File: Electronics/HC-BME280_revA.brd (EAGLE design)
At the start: 100 x 80 mm, 40 parts, among them SW1 SWITCH_SLIDE, T2 AO3401, U1 ATMEGA328-20P, U2 NRF24L01, U3 BME280, U4 OLED128X64, U5 BCO35

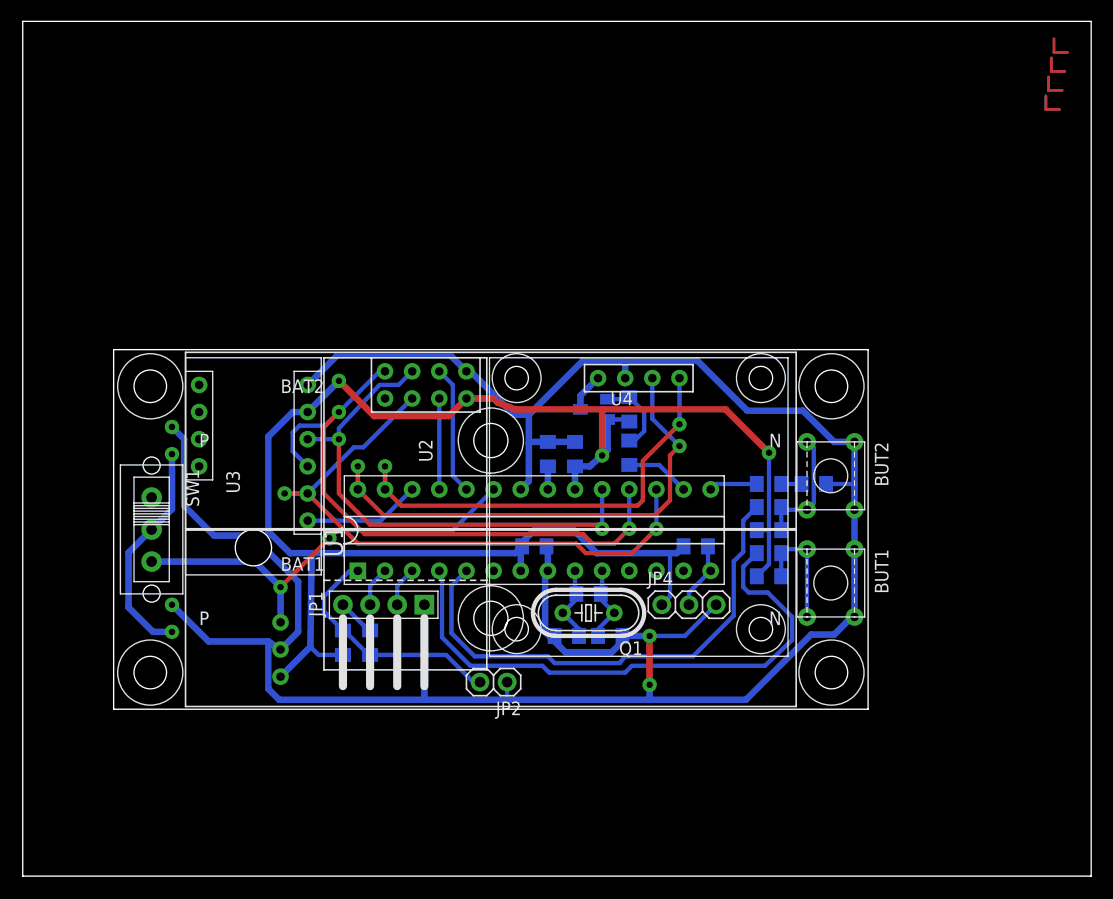
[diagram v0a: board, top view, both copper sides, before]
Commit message: modified: PCB
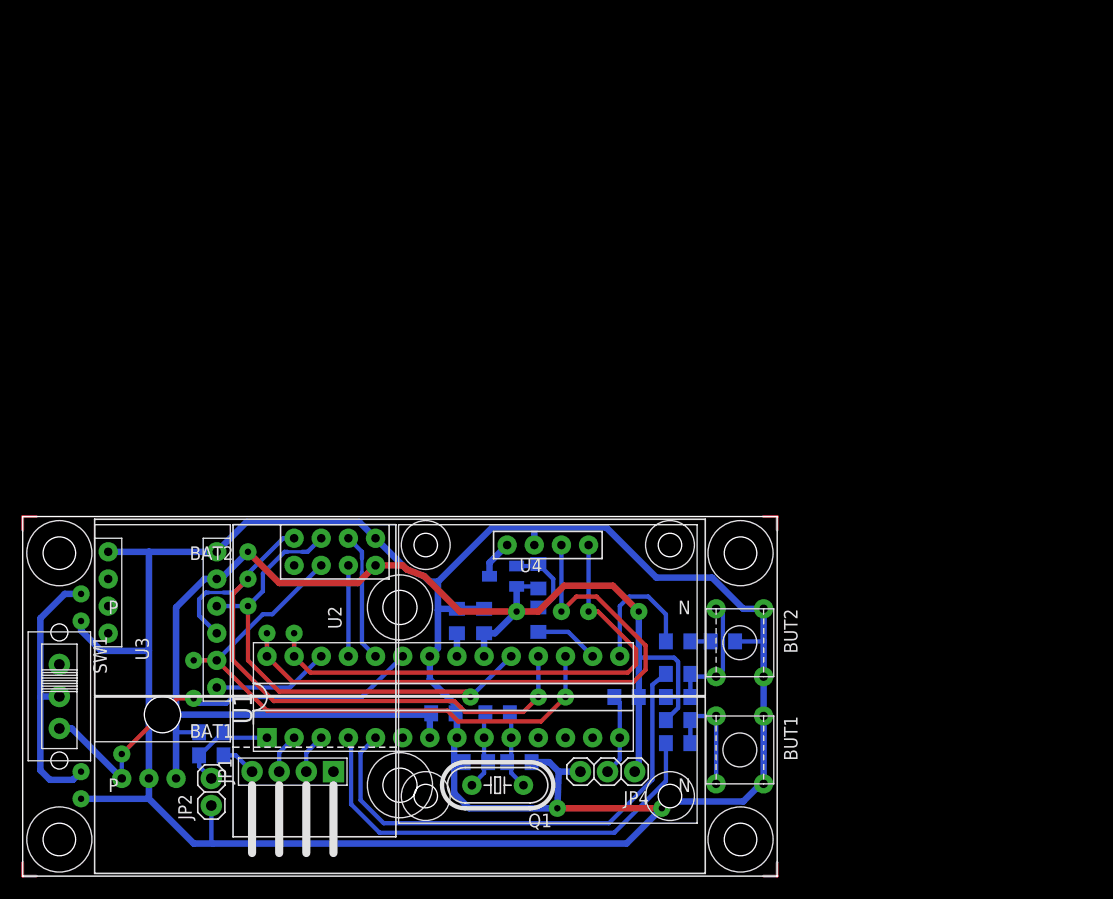
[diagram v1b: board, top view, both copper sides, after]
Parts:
- moved U$2 122.2 mm to (0.64, 0.64)
- moved U$3 104.5 mm to (0.64, 33.0), turned to 270 degrees
- moved U$4 76.5 mm to (70.0, 0.64), turned to 90 degrees
- moved U$1 52.3 mm to (70.0, 33.0), turned to 180 degrees
- moved JP2 28.3 mm to (17.7, 7.87), turned to 90 degrees
- moved R6 19.7 mm to (61.3, 12.4)
- moved Q1 18.2 mm to (44.5, 8.51)
- moved C4 18.2 mm to (17.7, 11.3), turned to 180 degrees
- moved SW1 17.8 mm to (3.43, 16.9)
- moved BAT2 17.8 mm to (35.3, 25.1)
- moved BUT2 17.8 mm to (67.4, 22.5)
- moved R2 17.8 mm to (48.3, 24.0)
- moved R3 17.8 mm to (48.3, 28.1)
- moved T2 17.8 mm to (45.0, 28.1)
- moved U$7 17.8 mm to (3.43, 30.2)
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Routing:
- net +3V3: track 156.0 -> 131.8 mm
- net GND: track 239.6 -> 255.2 mm
- net N$2: track 22.9 -> 10.1 mm
- net SCL: track 48.0 -> 60.1 mm
- net BUT1: track 53.3 -> 42.8 mm
- net SDA: track 42.1 -> 50.8 mm
- net LED: track 4.53 -> 12.6 mm
- net N$8: track 21.0 -> 25.3 mm
- net SCK: track 47.9 -> 46.1 mm
- net DS18B20_1: track 6.41 -> 7.67 mm
- net MISO: track 57.7 -> 58.6 mm
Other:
- board size 100 x 80 mm -> 70.6 x 33.7 mm

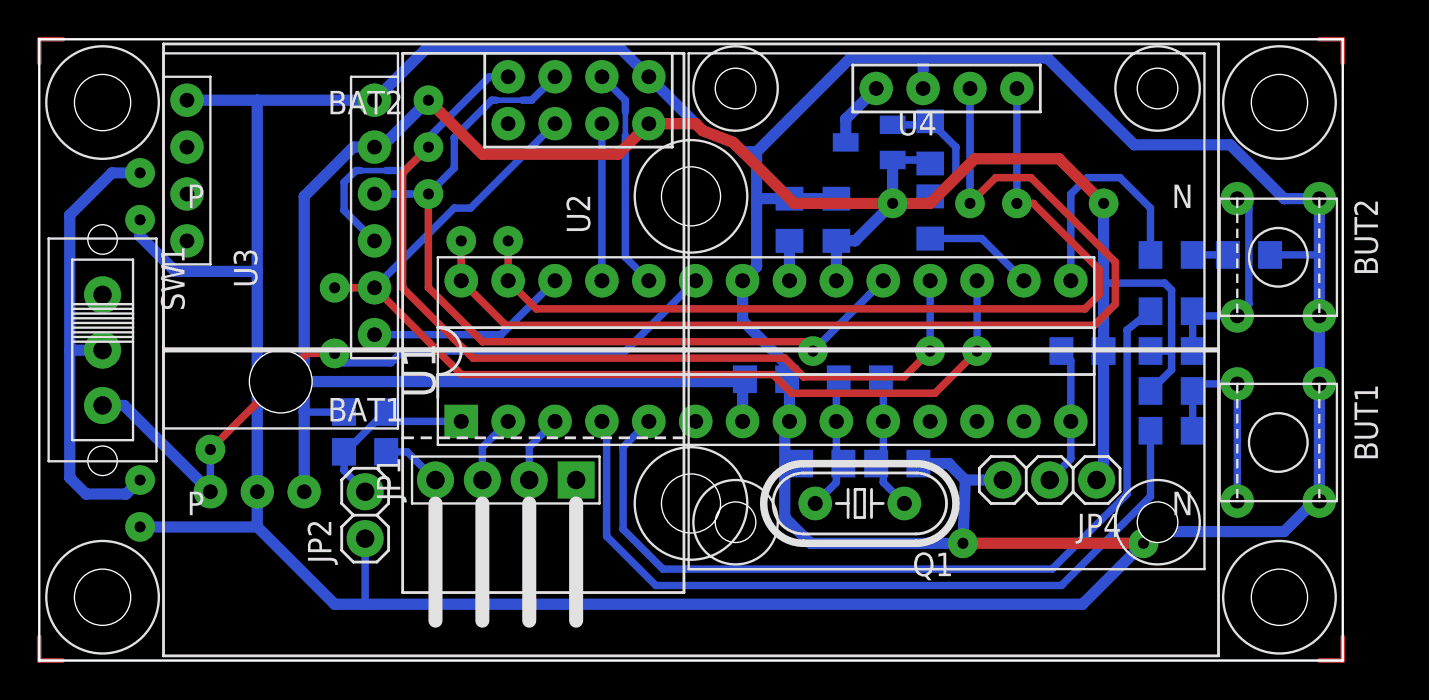
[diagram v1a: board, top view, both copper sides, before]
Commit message: modified: PCB - revA
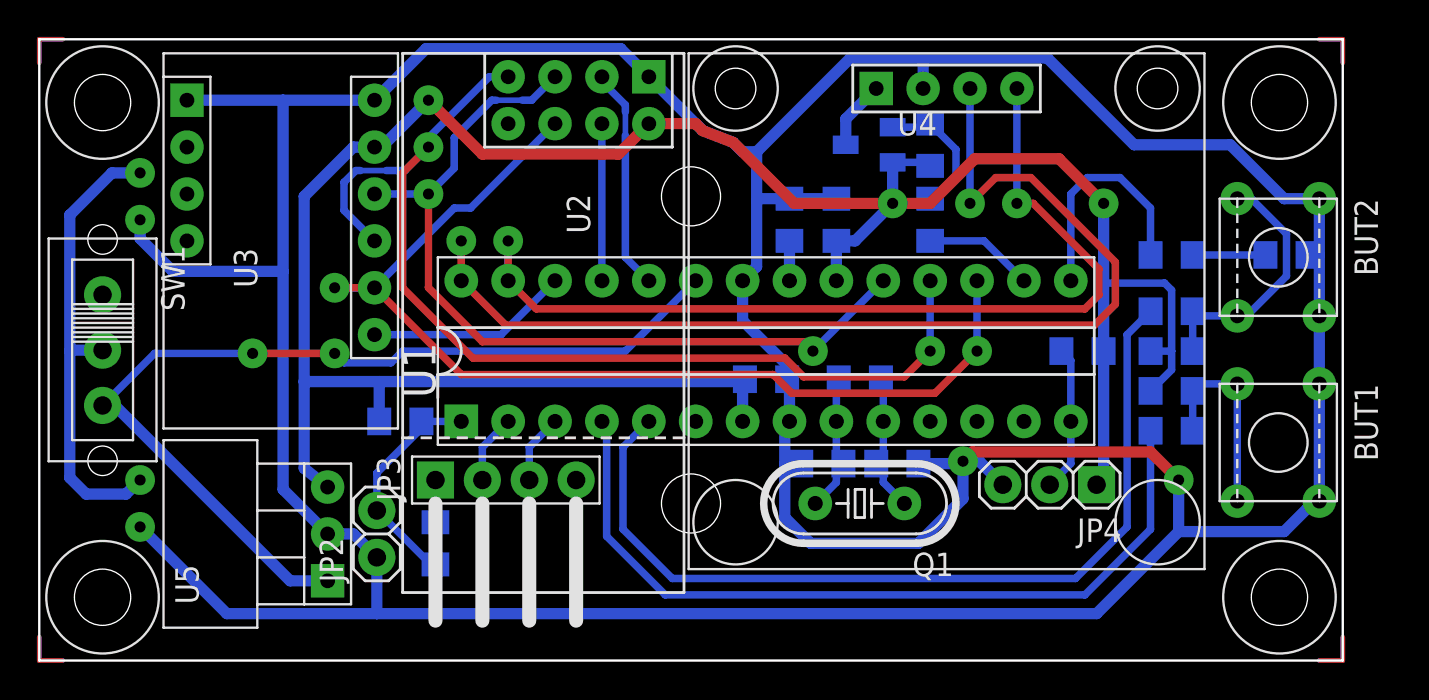
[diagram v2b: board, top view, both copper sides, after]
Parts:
- moved C4 6.25 mm to (21.5, 6.35), turned to 90 degrees
- moved U5 4.44 mm to (15.6, 6.86), flipped to the top, turned to 90 degrees
- moved LED1 2.03 mm to (67.6, 22.0)
- moved R1 1.97 mm to (19.6, 13.0)
- moved JP2 1.20 mm to (18.3, 6.86)
- moved JP4 0.25 mm to (54.7, 9.53)
- moved R2 0.13 mm to (48.3, 23.9)
- moved R3 0.13 mm to (48.3, 27.9)
- moved T2 0.13 mm to (45.0, 27.9)
- flipped BAT1 to the bottom, turned to 180 degrees
- flipped BAT2 to the bottom, turned to 180 degrees
- renumbered JP1 to JP3
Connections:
- net GND: now also JP3.4; no longer JP3.1
- net N$6: now also JP3.1; no longer JP3.4
- net RX: now also JP3.2; no longer JP3.3
- net TX: now also JP3.3; no longer JP3.2
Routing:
- net V_BAT: track 40.6 -> 51.5 mm
- net GND: track 255.2 -> 264.9 mm
- net N$2: track 10.1 -> 12.9 mm
- net N$10: track 11.6 -> 14.0 mm
- net N$11: track 1.90 -> 3.94 mm
- net BUT1: track 42.8 -> 44.3 mm
- net BUT2: track 46.8 -> 48.2 mm
- net N$6: track 3.30 -> 2.29 mm

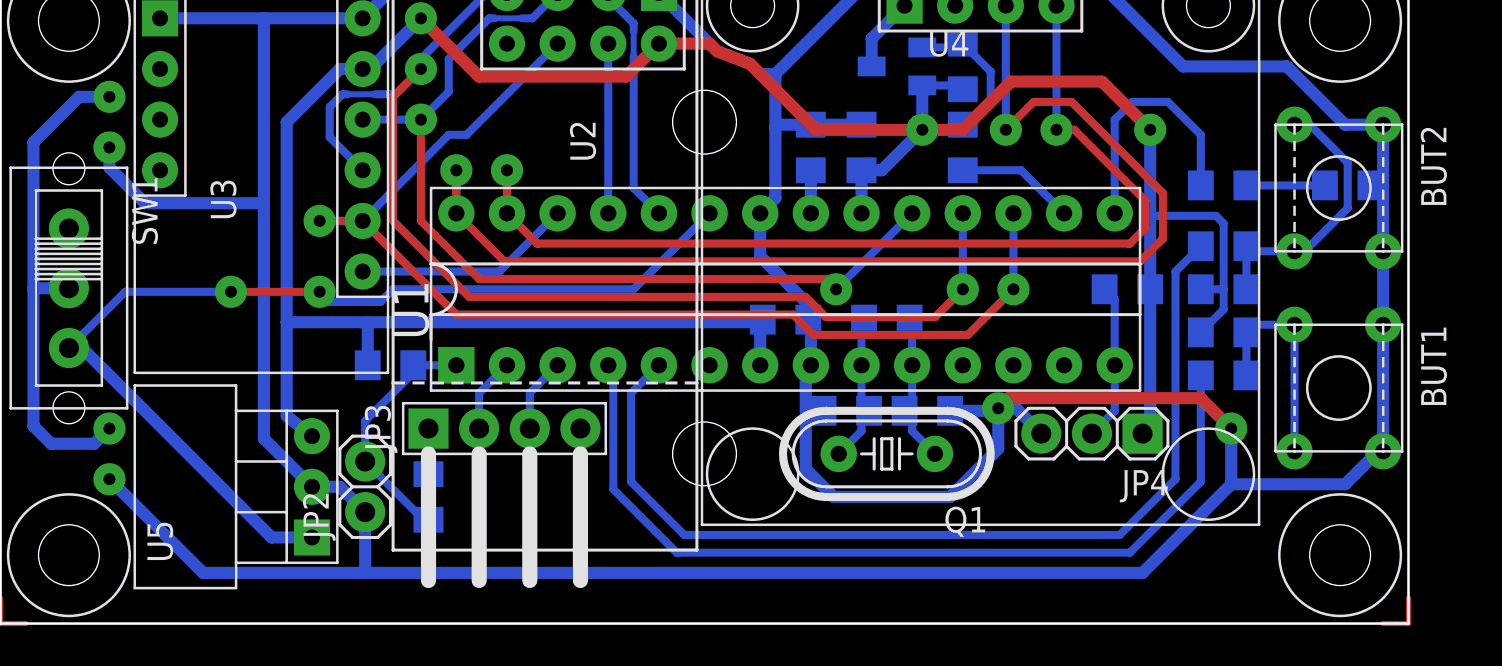
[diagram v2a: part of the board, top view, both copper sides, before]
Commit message: modified: minor changes in schematics and PCB
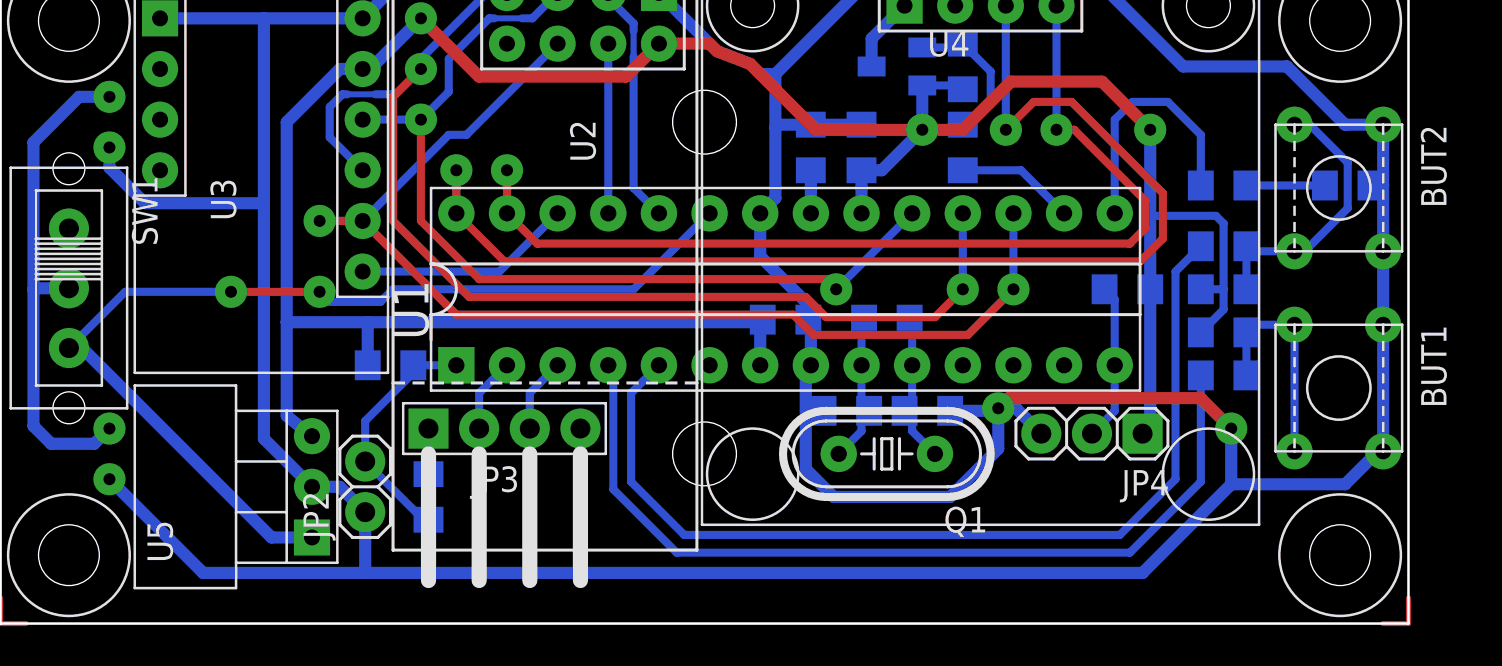
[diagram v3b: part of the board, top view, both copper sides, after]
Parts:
- JP2: value PINHD-2X1 -> PINHD2X1
- JP3: value (none) -> PINHD3X1
- LED1: value (none) -> green
- Q1: value (none) -> 16MHz
- R1: value (none) -> 4k7
